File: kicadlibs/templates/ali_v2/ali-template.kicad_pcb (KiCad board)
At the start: 4 copper layers, 85 x 76 mm, 71 parts, among them J1 Conn_02x01, J2 Conn_01x05, J3 USB_C_Receptacle_USB2.0_16P, J6 Screw_Terminal_01x02, J7 Conn_01x03, J8 Vertical Ethernet, SW1 SKRPANE010, U1 STM32H563RIV6, U2 AP2112K-3.3, U3 TJA1462ATK, U4 LAN8742AI, Y1 25 MHz, Y2 25 MHz

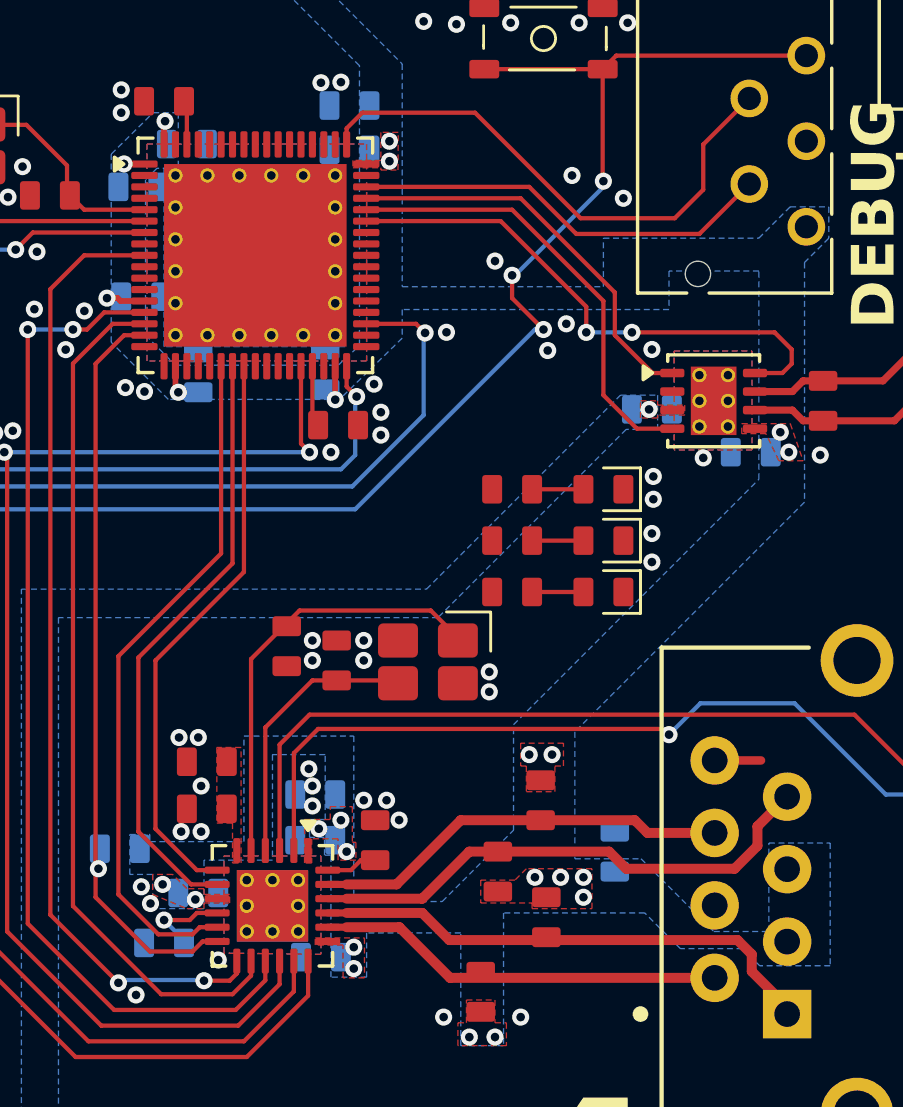
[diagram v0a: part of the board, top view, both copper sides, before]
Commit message: Begin prep for second board review
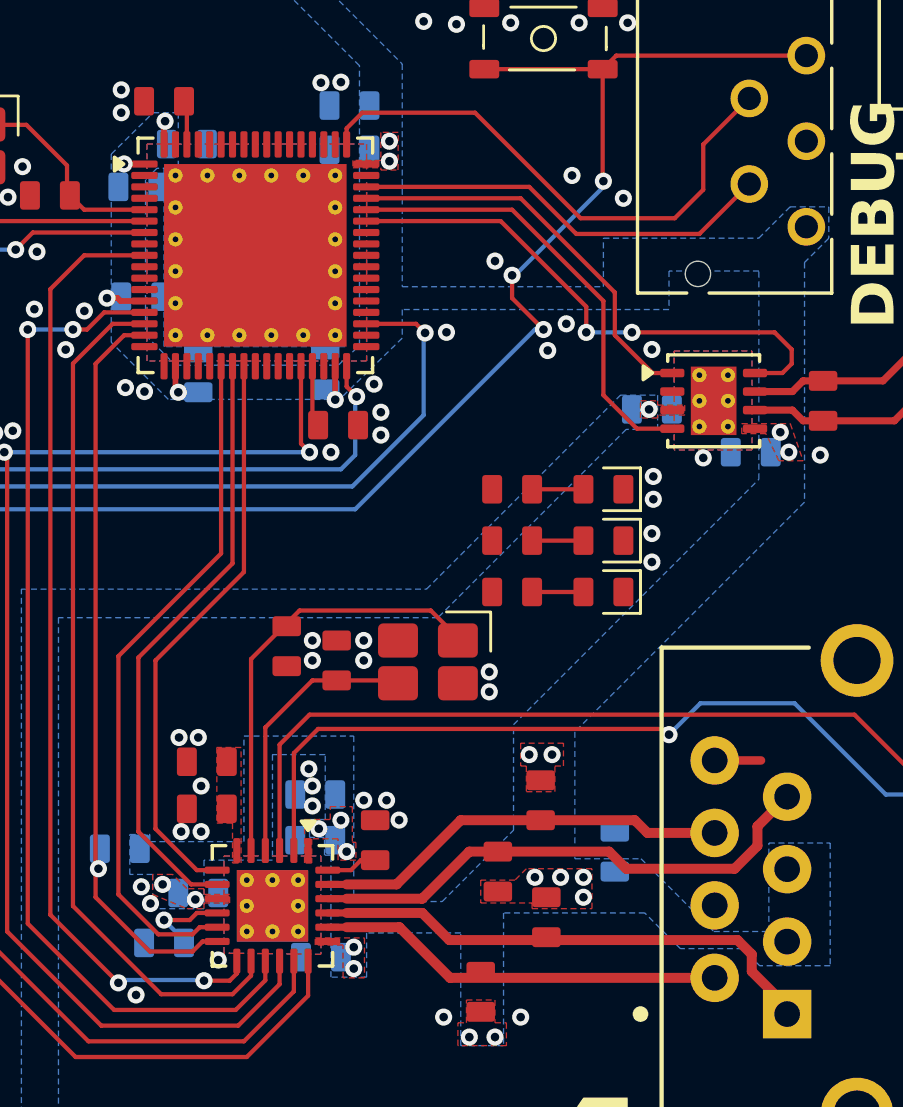
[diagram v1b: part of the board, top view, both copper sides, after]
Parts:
- R1, R2: value 4.7k -> 5.1k
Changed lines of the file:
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@@
 			)
 		)
-		(property "Value" "4.7k"
+		(property "Value" "5.1k"
 			(at 0 1 180)
 			(unlocked yes)
@@
 			)
 		)
-		(property "MPN" "RC0603FR-074K7L"
+		(property "MPN" "RC0603FR-075K1L"
 			(at 0 0 180)
 			(unlocked yes)
@@
 			(at -2.8 -2.8 90)
 			(size 0.5 0.5)
-			(drill 0.3)
+			(drill 0.2)
 			(layers "*.Cu")
 			(remove_unused_layers no)
@@
 			(at -2.8 -1.68 90)
 			(size 0.5 0.5)
-			(drill 0.3)
+			(drill 0.2)
 			(layers "*.Cu")
 			(remove_unused_layers no)
@@
 			(at -2.8 -0.56 90)
 			(size 0.5 0.5)
-			(drill 0.3)
+			(drill 0.2)
 			(layers "*.Cu")
 			(remove_unused_layers no)
@@
 			(at -2.8 0.56 90)
 			(size 0.5 0.5)
-			(drill 0.3)
+			(drill 0.2)
 			(layers "*.Cu")
 			(remove_unused_layers no)
@@
 			(at -2.8 1.68 90)
 			(size 0.5 0.5)
-			(drill 0.3)
+			(drill 0.2)
 			(layers "*.Cu")
 			(remove_unused_layers no)
@@
 			(at -2.8 2.8 90)
 			(size 0.5 0.5)
-			(drill 0.3)
+			(drill 0.2)
 			(property pad_prop_heatsink)
 			(layers "*.Cu")
@@
 			(at -1.68 -2.8)
 			(size 0.5 0.5)
-			(drill 0.3)
+			(drill 0.2)
 			(layers "*.Cu")
 			(remove_unused_layers no)
@@
 			(at -1.68 2.8 180)
 			(size 0.5 0.5)
-			(drill 0.3)
+			(drill 0.2)
 			(layers "*.Cu")
 			(remove_unused_layers no)
@@
 			(at -0.56 -2.8)
 			(size 0.5 0.5)
-			(drill 0.3)
+			(drill 0.2)
 			(layers "*.Cu")
 			(remove_unused_layers no)
@@
 			(at -0.56 2.8 180)
 			(size 0.5 0.5)
-			(drill 0.3)
+			(drill 0.2)
 			(layers "*.Cu")
 			(remove_unused_layers no)
@@
 			(at 0.56 -2.8)
 			(size 0.5 0.5)
-			(drill 0.3)
+			(drill 0.2)
 			(layers "*.Cu")
 			(remove_unused_layers no)
@@
 			(at 0.56 2.8 180)
 			(size 0.5 0.5)
-			(drill 0.3)
+			(drill 0.2)
 			(layers "*.Cu")
 			(remove_unused_layers no)
@@
 			(at 1.68 -2.8)
 			(size 0.5 0.5)
-			(drill 0.3)
+			(drill 0.2)
 			(layers "*.Cu")
 			(remove_unused_layers no)
@@
 			(at 1.68 2.8 180)
 			(size 0.5 0.5)
-			(drill 0.3)
+			(drill 0.2)
 			(layers "*.Cu")
 			(remove_unused_layers no)
@@
 			(at 2.8 -2.8 270)
 			(size 0.5 0.5)
-			(drill 0.3)
+			(drill 0.2)
 			(property pad_prop_heatsink)
 			(layers "*.Cu")
@@
 			(at 2.8 -1.68 270)
 			(size 0.5 0.5)
-			(drill 0.3)
+			(drill 0.2)
 			(layers "*.Cu")
 			(remove_unused_layers no)
@@
 			(at 2.8 -0.56 270)
 			(size 0.5 0.5)
-			(drill 0.3)
+			(drill 0.2)
 			(layers "*.Cu")
 			(remove_unused_layers no)
@@
 			(at 2.8 0.56 270)
 			(size 0.5 0.5)
-			(drill 0.3)
+			(drill 0.2)
 			(layers "*.Cu")
 			(remove_unused_layers no)
@@
 			(at 2.8 1.68 270)
 			(size 0.5 0.5)
-			(drill 0.3)
+			(drill 0.2)
 			(layers "*.Cu")
 			(remove_unused_layers no)
@@
 			(at 2.8 2.8 180)
 			(size 0.5 0.5)
-			(drill 0.3)
+			(drill 0.2)
 			(property pad_prop_heatsink)
 			(layers "*.Cu")
@@
 			(at -0.5 -0.9)
 			(size 0.5 0.5)
-			(drill 0.3)
+			(drill 0.2)
 			(layers "*.Cu")
 			(remove_unused_layers no)
@@
 			(at -0.5 0)
 			(size 0.5 0.5)
-			(drill 0.3)
+			(drill 0.2)
 			(layers "*.Cu")
 			(remove_unused_layers no)
@@
 			(at -0.5 0.9)
 			(size 0.5 0.5)
-			(drill 0.3)
+			(drill 0.2)
 			(layers "*.Cu")
 			(remove_unused_layers no)
@@
 			(at 0.5 -0.9)
 			(size 0.5 0.5)
-			(drill 0.3)
+			(drill 0.2)
 			(layers "*.Cu")
 			(remove_unused_layers no)
@@
 			(at 0.5 0)
 			(size 0.5 0.5)
-			(drill 0.3)
+			(drill 0.2)
 			(layers "*.Cu")
 			(remove_unused_layers no)
@@
 			(at 0.5 0.9)
 			(size 0.5 0.5)
-			(drill 0.3)
+			(drill 0.2)
 			(layers "*.Cu")
 			(remove_unused_layers no)
@@
 			)
 		)
-		(property "Value" "4.7k"
+		(property "Value" "5.1k"
 			(at 0 1 180)
 			(unlocked yes)
@@
 			)
 		)
-		(property "MPN" "RC0603FR-074K7L"
+		(property "MPN" "RC0603FR-075K1L"
 			(at 0 0 180)
 			(unlocked yes)
@@
 			(at -0.9 -0.9 270)
 			(size 0.5 0.5)
-			(drill 0.3)
+			(drill 0.2)
 			(property pad_prop_heatsink)
 			(layers "*.Cu")
@@
 			(at -0.9 0 270)
 			(size 0.5 0.5)
-			(drill 0.3)
+			(drill 0.2)
 			(property pad_prop_heatsink)
 			(layers "*.Cu")
@@
 			(at -0.9 0.9 270)
 			(size 0.5 0.5)
-			(drill 0.3)
+			(drill 0.2)
 			(property pad_prop_heatsink)
 			(layers "*.Cu")
@@
 			(at 0 -0.9 270)
 			(size 0.5 0.5)
-			(drill 0.3)
+			(drill 0.2)
 			(property pad_prop_heatsink)
 			(layers "*.Cu")
@@
 			(at 0 0.9 270)
 			(size 0.5 0.5)
-			(drill 0.3)
+			(drill 0.2)
 			(property pad_prop_heatsink)
 			(layers "*.Cu")
@@
 			(at 0.9 -0.9 270)
 			(size 0.5 0.5)
-			(drill 0.3)
+			(drill 0.2)
 			(property pad_prop_heatsink)
 			(layers "*.Cu")
@@
 			(at 0.9 0 270)
 			(size 0.5 0.5)
-			(drill 0.3)
+			(drill 0.2)
 			(property pad_prop_heatsink)
 			(layers "*.Cu")
@@
 			(at 0.9 0.9 270)
 			(size 0.5 0.5)
-			(drill 0.3)
+			(drill 0.2)
 			(property pad_prop_heatsink)
 			(layers "*.Cu")
